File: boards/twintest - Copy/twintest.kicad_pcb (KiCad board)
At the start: 2 copper layers, 138 x 111 mm, 64 parts, among them SW1 Switch, U1 Nice_Nano_V2, U2 Nice_Nano_V2

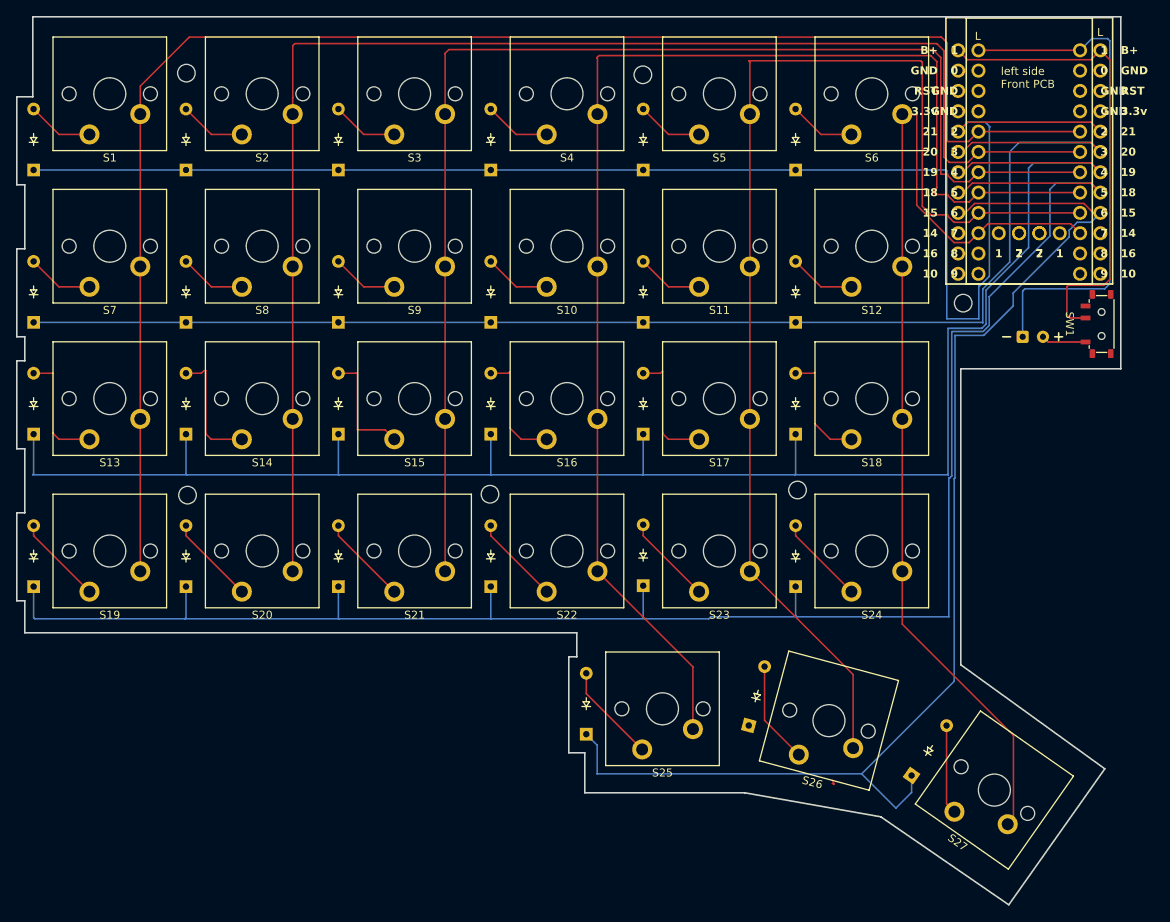
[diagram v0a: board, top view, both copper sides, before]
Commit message: test
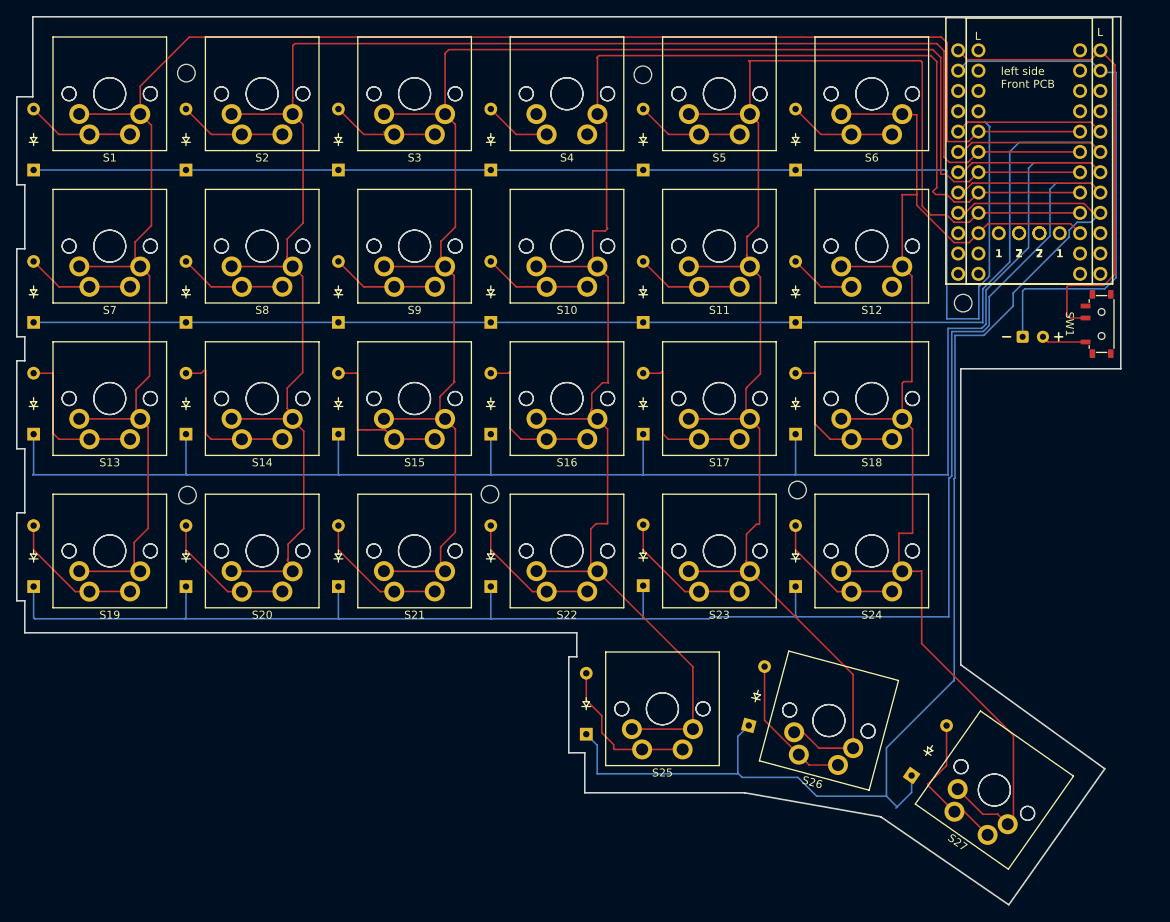
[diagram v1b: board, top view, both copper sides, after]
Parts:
- added S1: Keyswitch, ScottoKeebs_MX:MX_PCB_1.00u, B.Cu at (47.6, 47.6)
- added S10: Keyswitch, ScottoKeebs_MX:MX_PCB_1.00u, B.Cu at (104.8, 66.7)
- added S11: Keyswitch, ScottoKeebs_MX:MX_PCB_1.00u, B.Cu at (123.8, 66.7)
- added S12: Keyswitch, ScottoKeebs_MX:MX_PCB_1.00u, B.Cu at (142.9, 66.7)
- added S13: Keyswitch, ScottoKeebs_MX:MX_PCB_1.00u, B.Cu at (47.6, 85.7)
- added S14: Keyswitch, ScottoKeebs_MX:MX_PCB_1.00u, B.Cu at (66.7, 85.7)
- added S15: Keyswitch, ScottoKeebs_MX:MX_PCB_1.00u, B.Cu at (85.7, 85.7)
- added S16: Keyswitch, ScottoKeebs_MX:MX_PCB_1.00u, B.Cu at (104.8, 85.7)
- added S17: Keyswitch, ScottoKeebs_MX:MX_PCB_1.00u, B.Cu at (123.8, 85.7)
- added S18: Keyswitch, ScottoKeebs_MX:MX_PCB_1.00u, B.Cu at (142.9, 85.7)
- added S19: Keyswitch, ScottoKeebs_MX:MX_PCB_1.00u, B.Cu at (47.6, 104.8)
- added S2: Keyswitch, ScottoKeebs_MX:MX_PCB_1.00u, B.Cu at (66.7, 47.6)
- added S20: Keyswitch, ScottoKeebs_MX:MX_PCB_1.00u, B.Cu at (66.7, 104.8)
- added S21: Keyswitch, ScottoKeebs_MX:MX_PCB_1.00u, B.Cu at (85.7, 104.8)
- added S22: Keyswitch, ScottoKeebs_MX:MX_PCB_1.00u, B.Cu at (104.8, 104.8)
- added S23: Keyswitch, ScottoKeebs_MX:MX_PCB_1.00u, B.Cu at (123.8, 104.8)
- added S24: Keyswitch, ScottoKeebs_MX:MX_PCB_1.00u, B.Cu at (142.9, 104.8)
- added S25: Keyswitch, ScottoKeebs_MX:MX_PCB_1.00u, B.Cu at (116.7, 124.5)
- added S26: Keyswitch, ScottoKeebs_MX:MX_PCB_1.00u, B.Cu at (137.5, 126.0)
- added S27: Keyswitch, ScottoKeebs_MX:MX_PCB_1.00u, B.Cu at (158.2, 134.6)
- added S3: Keyswitch, ScottoKeebs_MX:MX_PCB_1.00u, B.Cu at (85.7, 47.6)
- added S4: Keyswitch, ScottoKeebs_MX:MX_PCB_1.00u, B.Cu at (104.8, 47.6)
- added S5: Keyswitch, ScottoKeebs_MX:MX_PCB_1.00u, B.Cu at (123.8, 47.6)
- added S6: Keyswitch, ScottoKeebs_MX:MX_PCB_1.00u, B.Cu at (142.9, 47.6)
- added S7: Keyswitch, ScottoKeebs_MX:MX_PCB_1.00u, B.Cu at (47.6, 66.7)
- added S8: Keyswitch, ScottoKeebs_MX:MX_PCB_1.00u, B.Cu at (66.7, 66.7)
- added S9: Keyswitch, ScottoKeebs_MX:MX_PCB_1.00u, B.Cu at (85.7, 66.7)
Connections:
- SW1 pad 1: Net-(BT2-+) -> battery +
- SW1 pad 2: battery + -> Net-(BT2-+)
- U1 pad 1: battery - -> unconnected-(U1-Pad1)
- U1 pad 23: unconnected-(U1-GND-Pad23) -> battery -
- U2 pad 1: battery - -> unconnected-(U2-Pad1)
- U2 pad 23: unconnected-(U2-GND-Pad23) -> battery -
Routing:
- net collumn 5: track 152.3 -> 195.6 mm
- net collumn 4: track 167.9 -> 205.6 mm
- net collumn 6: track 131.8 -> 167.7 mm
- net collumn 2: track 178.7 -> 214.3 mm
- net collumn 1: track 194.5 -> 229.5 mm
- net collumn 3: track 160.4 -> 195.4 mm
- net row 5: track 153.9 -> 162.2 mm
- net Net-(D27-A): track 11.2 -> 18.5 mm
- net Net-(D25-A): track 12.4 -> 19.5 mm
- net Net-(D24-A): track 11.1 -> 17.3 mm
- net Net-(D22-A): track 11.1 -> 17.3 mm
- net Net-(D19-A): track 11.1 -> 17.3 mm
- net Net-(D20-A): track 11.1 -> 17.3 mm
- net Net-(D23-A): track 11.3 -> 17.4 mm
- net Net-(D21-A): track 11.1 -> 17.2 mm
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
